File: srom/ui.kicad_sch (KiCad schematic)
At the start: 17 parts, among them J301 Conn_01x10_Female, J303 Conn_01x03_Female, SW301 SW_MEC_5E, SW302 RotaryEncoder_Switch, SW303 SW_MEC_5E, U301 Pico-3 UI

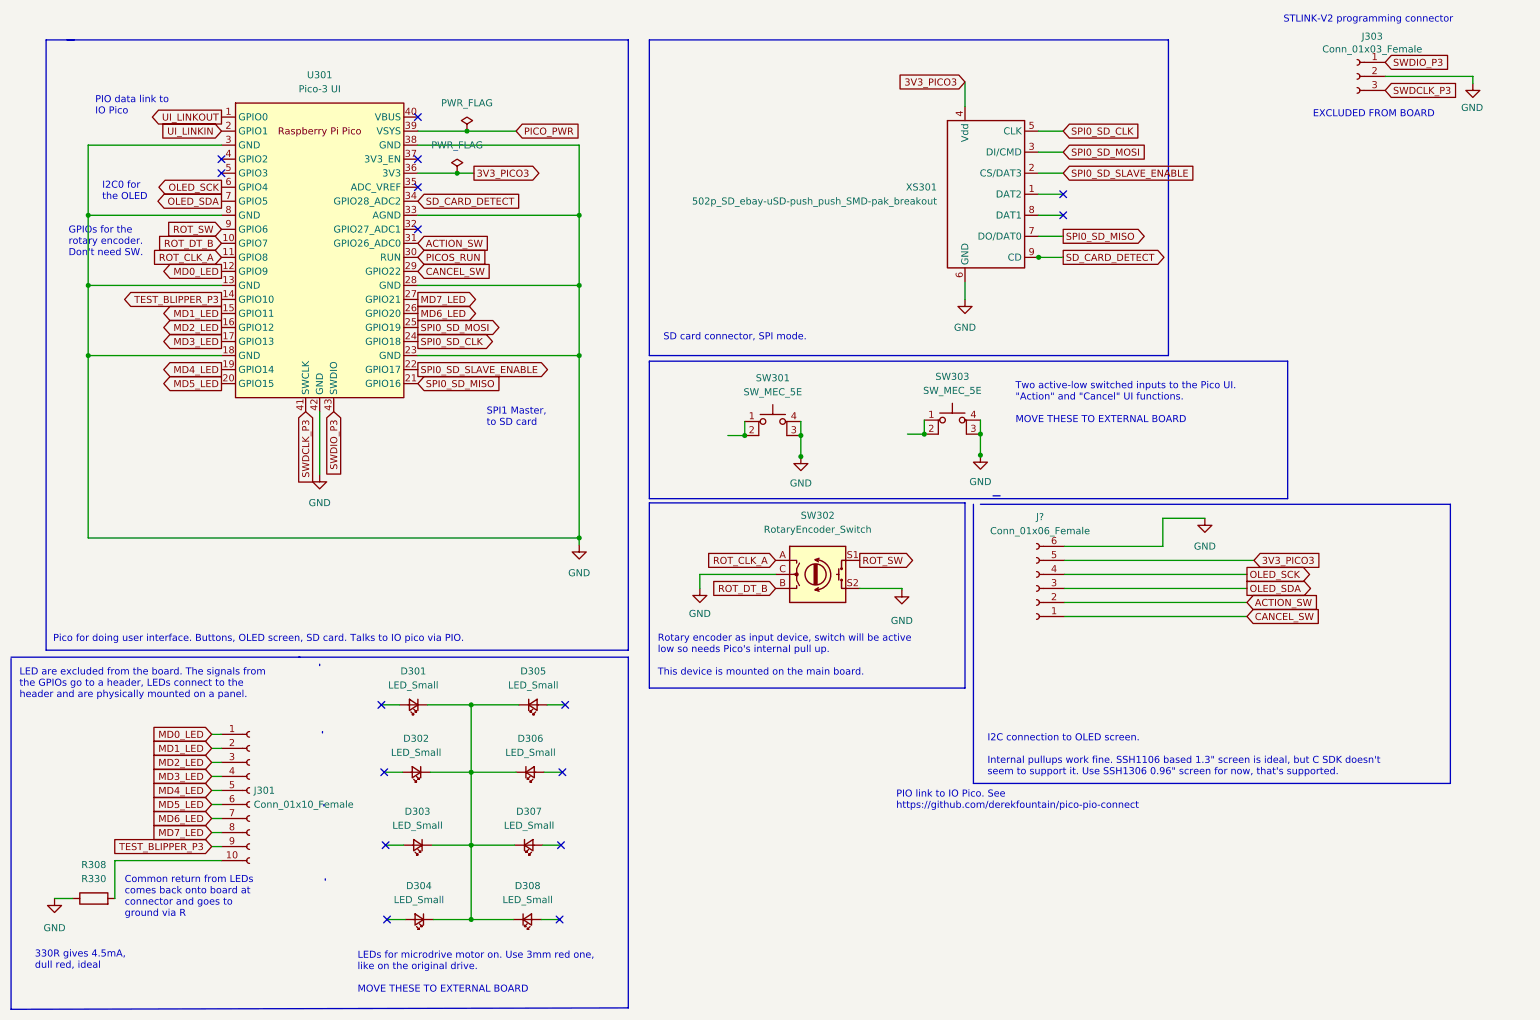
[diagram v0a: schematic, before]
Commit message: first draft of daughterboard taking shape
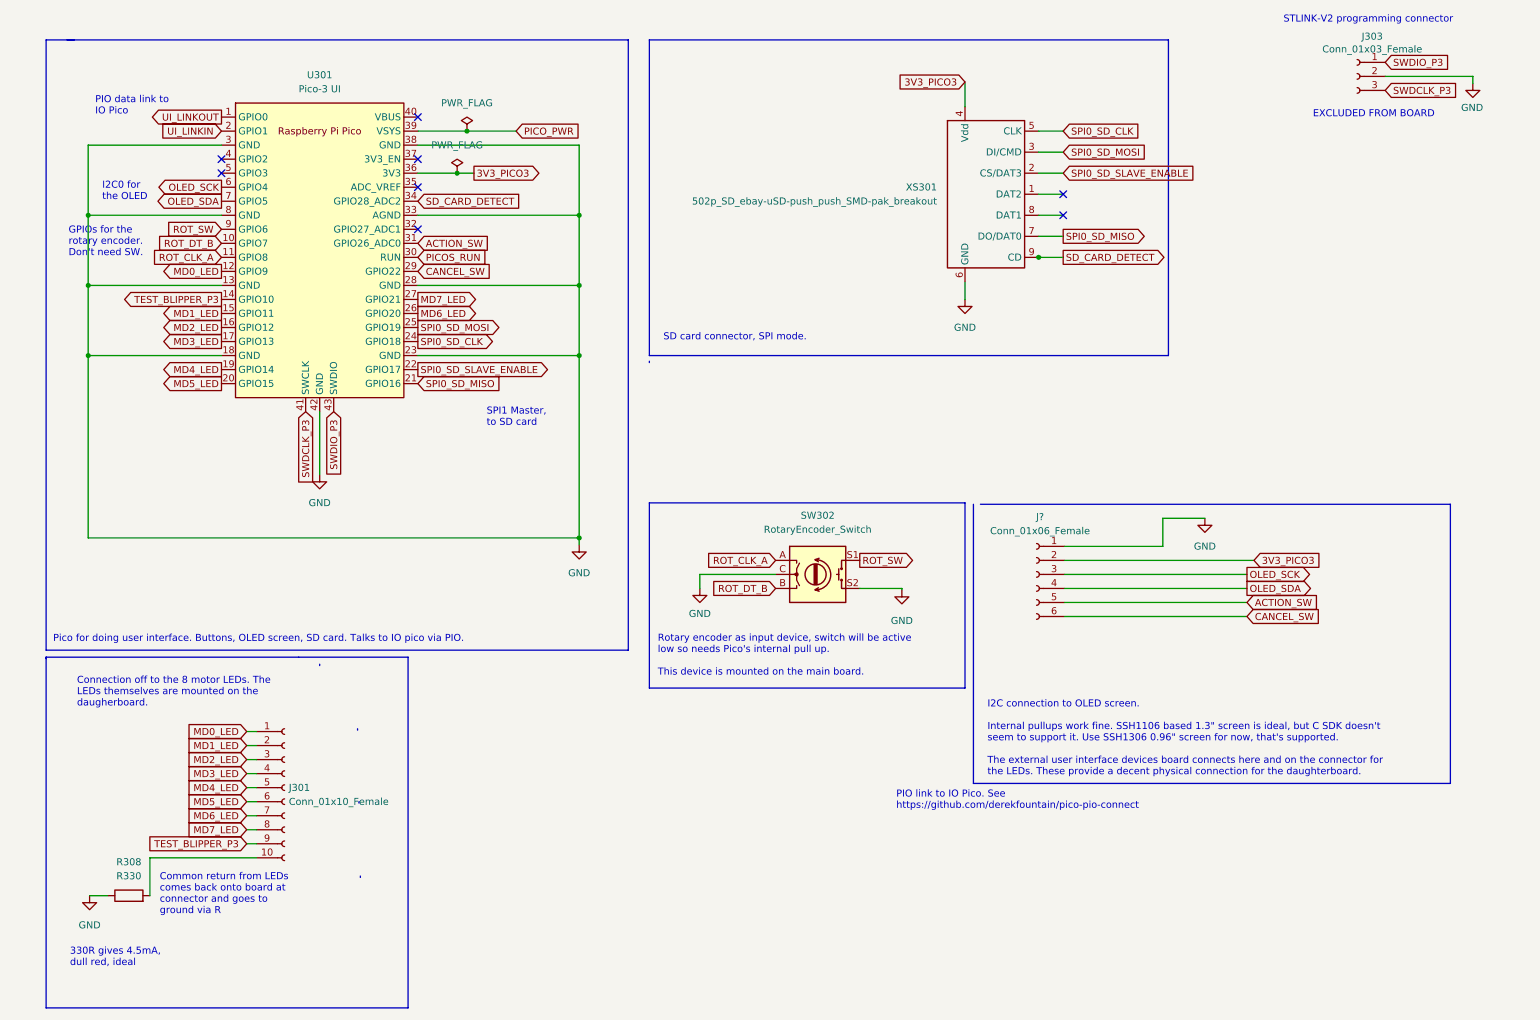
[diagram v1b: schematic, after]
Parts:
- removed D301, D302, D303, D304, D305, D306, D307, D308: LED_Small, LED_THT:LED_D3.0mm, symbol Device:LED_Small
- removed SW301, SW303: SW_MEC_5E, Button_Switch_THT:SW_PUSH_6mm_H4.3mm, symbol Switch:SW_MEC_5E
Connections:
- net 3V3_PICO3: now also J?.2 (Pin_2); no longer J?.5 (Pin_5)
- net ACTION_SW: now also J?.5 (Pin_5); no longer J?.2 (Pin_2)
- net CANCEL_SW: now also J?.6 (Pin_6); no longer J?.1 (Pin_1)
- net GND: now also J?.1 (Pin_1); no longer J?.6 (Pin_6)
- net OLED_SCK: now also J?.3 (Pin_3); no longer J?.4 (Pin_4)
- net OLED_SDA: now also J?.4 (Pin_4); no longer J?.3 (Pin_3)
- no-connect marks 16 -> 8
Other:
- note added: "Connection off to the 8 motor LEDs. The LEDs themselves are mounted on the daugherboard."
- note added: "I2C connection to OLED screen. Internal pullups work fine. SSH1106 based 1.3" screen is ideal, but C SDK doesn't seem to support it. Use SSH1306 0.96" screen for now, that's supported. The external user interface devices board connects here and on the connector for the LEDs. These provide a decent physical connection for the daughterboard."
- note removed: "I2C connection to OLED screen. Internal pullups work fine. SSH1106 based 1.3" screen is ideal, but C SDK doesn't seem to support it. Use SSH1306 0.96" screen for now, that's supported."
- note removed: "LED are excluded from the board. The signals from the GPIOs go to a header, LEDs connect to the header and are physically mounted on a panel."
- note removed: "LEDs for microdrive motor on. Use 3mm red one, like on the original drive. MOVE THESE TO EXTERNAL BOARD"
- note removed: "Two active-low switched inputs to the Pico UI. "Action" and "Cancel" UI functions. MOVE THESE TO EXTERNAL BOARD"
- moved on the sheet: J301, J?, R308
